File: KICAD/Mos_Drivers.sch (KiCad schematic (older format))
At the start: 15 parts, among them U12 UCC27284-Q1

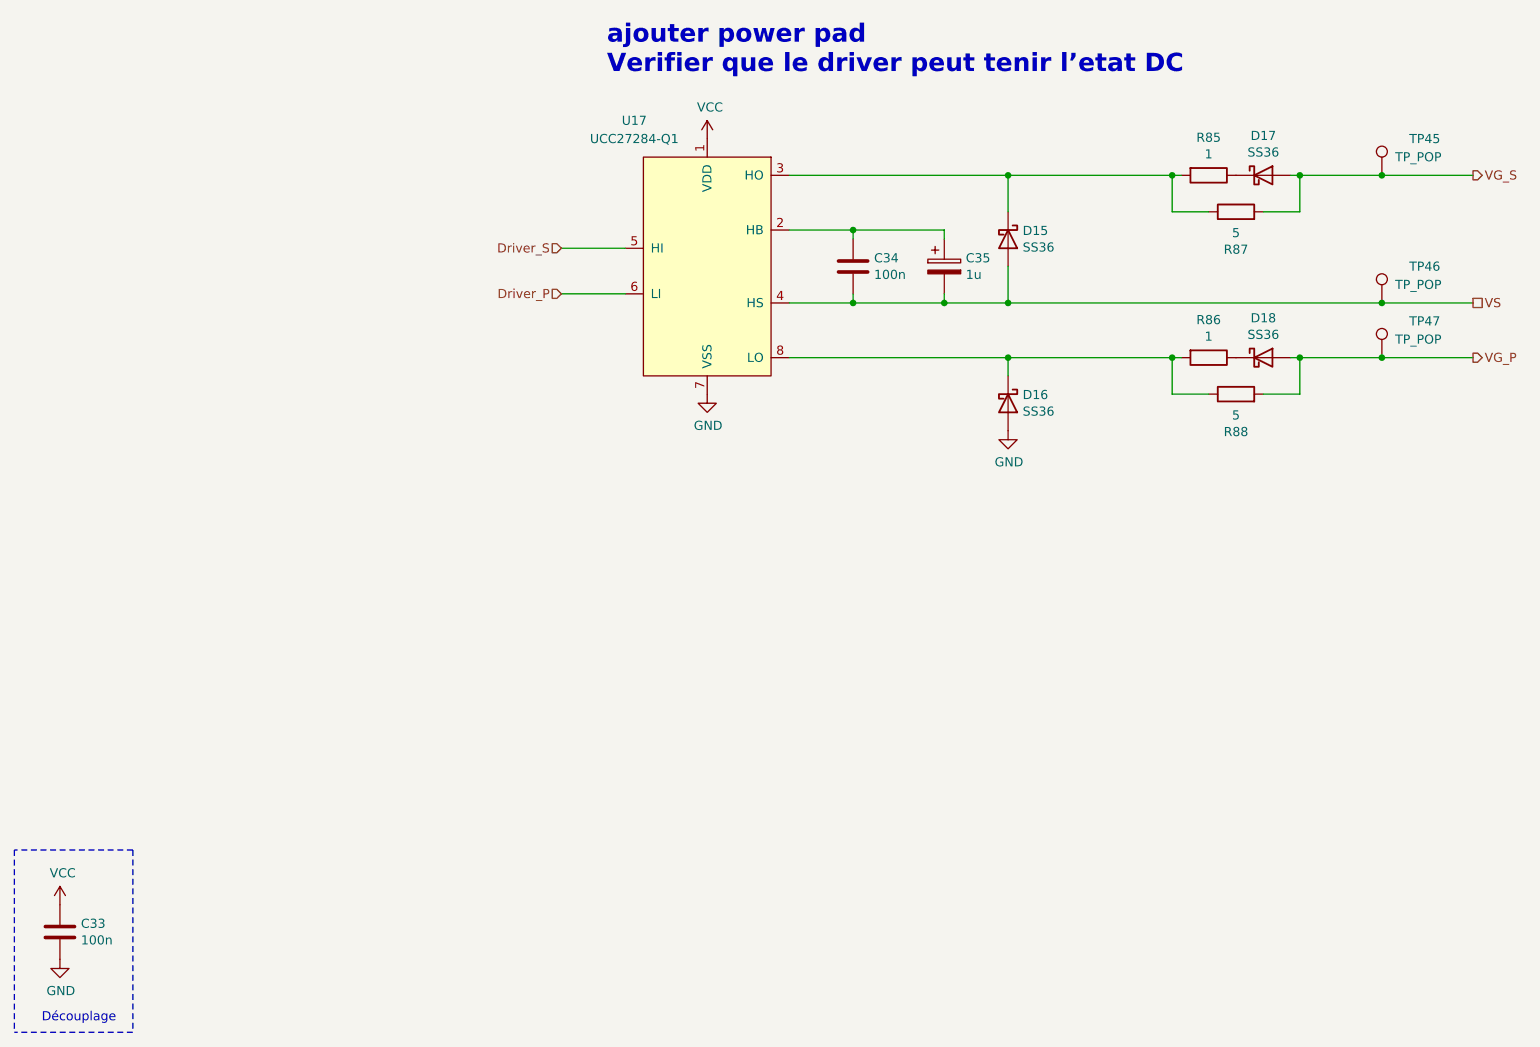
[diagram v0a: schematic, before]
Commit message: route + work on djd
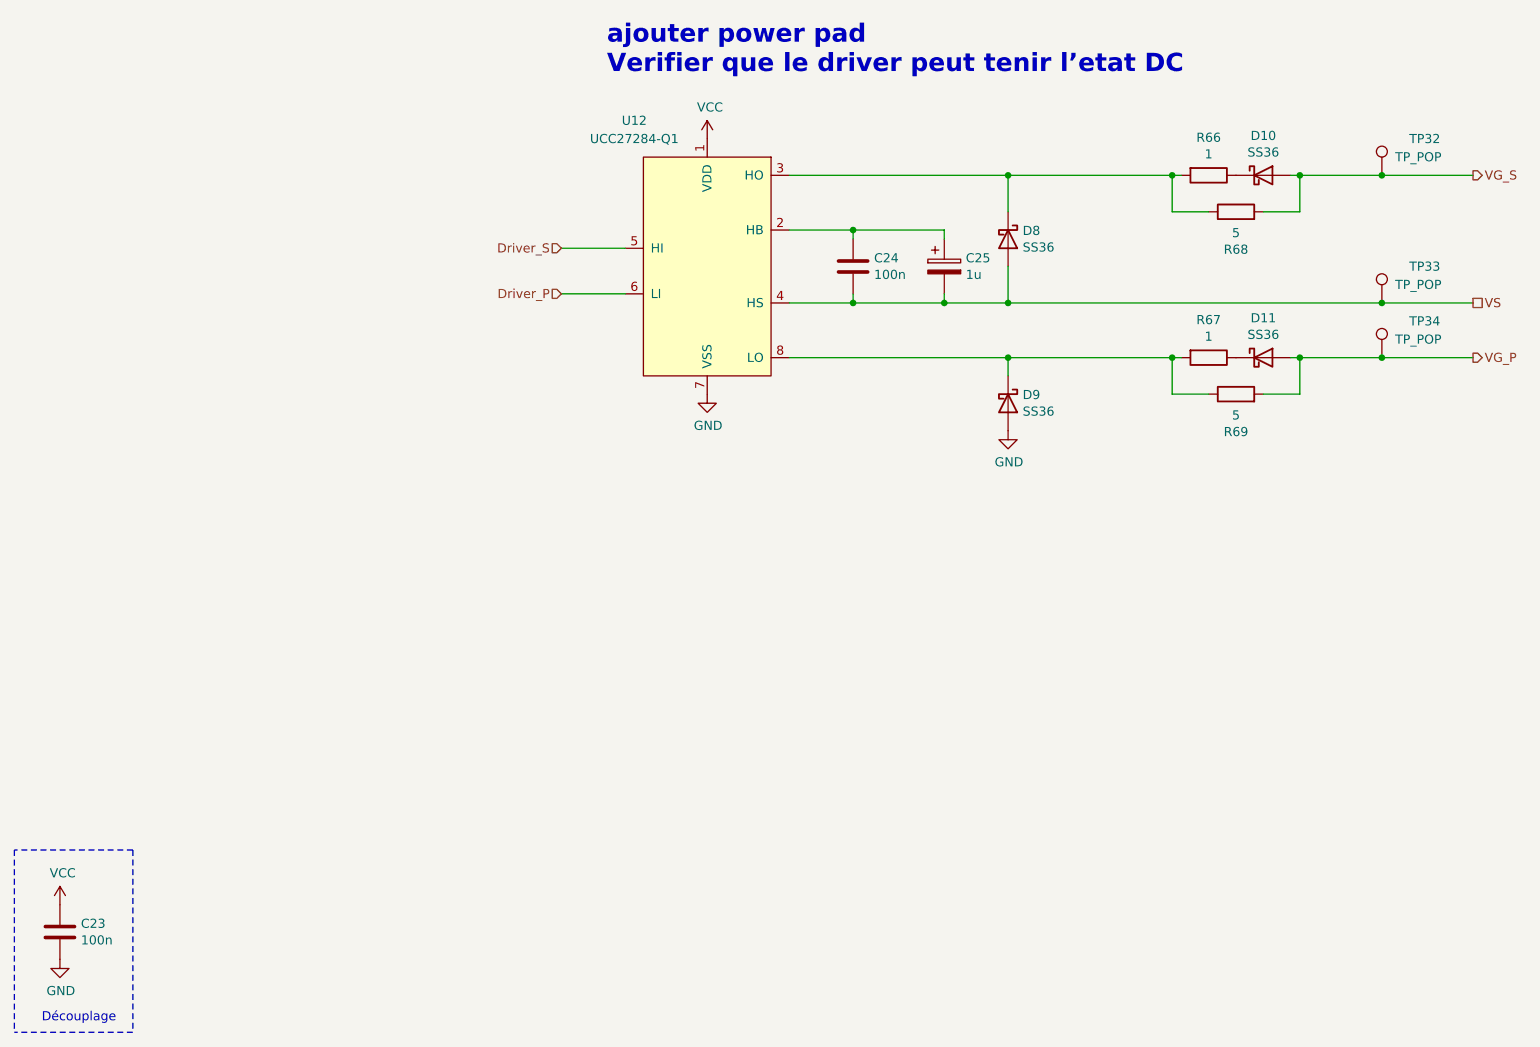
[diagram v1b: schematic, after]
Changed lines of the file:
@@
 $Descr A4 11693 8268
 encoding utf-8
-Sheet 16 17
+Sheet 12 17
 Title "SESAME"
 Date ""
@@
 AR Path="/61996C9F/612BC387" Ref="C?"  Part="1"
 AR Path="/619A00BB/612BC387" Ref="C33"  Part="1"
-F 0 "C33" H 965 7146 50  0000 L CNN
+F 0 "C23" H 965 7146 50  0000 L CNN
 F 1 "100n" H 965 7055 50  0000 L CNN
 F 2 "Capacitor_SMD:C_0805_2012Metric_Pad1.15x1.40mm_HandSolder" H 888 6950 50  0001 C CNN
@@
 AR Path="/61996C9F/612C31FB" Ref="D?"  Part="1"
 AR Path="/619A00BB/612C31FB" Ref="D15"  Part="1"
-F 0 "D15" V 6004 3380 50  0000 L CNN
+F 0 "D8" V 6004 3380 50  0000 L CNN
 F 1 "SS36" V 6095 3380 50  0000 L CNN
 F 2 "Diode_SMD:D_SMA_Handsoldering" H 6050 3300 50  0001 C CNN
@@
 AR Path="/61996C9F/6154F3B3" Ref="TP?"  Part="1"
 AR Path="/619A00BB/6154F3B3" Ref="TP46"  Part="1"
-F 0 "TP46" H 8250 3850 50  0000 L CNN
+F 0 "TP33" H 8250 3850 50  0000 L CNN
 F 1 "TP_POP" H 8300 3750 50  0000 C CNN
 F 2 "TestPoint:TestPoint_Loop_D1.80mm_Drill1.0mm_Beaded" H 8300 3650 50  0001 C CNN
@@
 AR Path="/61996C9F/61556ADA" Ref="TP?"  Part="1"
 AR Path="/619A00BB/61556ADA" Ref="TP47"  Part="1"
-F 0 "TP47" H 8250 4150 50  0000 L CNN
+F 0 "TP34" H 8250 4150 50  0000 L CNN
 F 1 "TP_POP" H 8300 4050 50  0000 C CNN
 F 2 "TestPoint:TestPoint_Loop_D1.80mm_Drill1.0mm_Beaded" H 8300 3950 50  0001 C CNN
@@
 AR Path="/61996C9F/61556D55" Ref="TP?"  Part="1"
 AR Path="/619A00BB/61556D55" Ref="TP45"  Part="1"
-F 0 "TP45" H 8250 3150 50  0000 L CNN
+F 0 "TP32" H 8250 3150 50  0000 L CNN
 F 1 "TP_POP" H 8300 3050 50  0000 C CNN
 F 2 "TestPoint:TestPoint_Loop_D1.80mm_Drill1.0mm_Beaded" H 8300 2950 50  0001 C CNN
@@
 AR Path="/61996C9F/615F8500" Ref="U?"  Part="1"
 AR Path="/619A00BB/615F8500" Ref="U17"  Part="1"
-F 0 "U17" H 4000 4250 50  0000 C CNN
+F 0 "U12" H 4000 4250 50  0000 C CNN
 F 1 "UCC27284-Q1" H 4000 4150 50  0000 C CNN
 F 2 "Package_SO:SOIC-8_3.9x4.9mm_P1.27mm" H 4400 3450 50  0001 C CNN
@@
 AR Path="/61996C9F/617A570A" Ref="D?"  Part="1"
 AR Path="/619A00BB/617A570A" Ref="D16"  Part="1"
-F 0 "D16" V 6004 4280 50  0000 L CNN
+F 0 "D9" V 6004 4280 50  0000 L CNN
 F 1 "SS36" V 6095 4280 50  0000 L CNN
 F 2 "Diode_SMD:D_SMA_Handsoldering" H 6050 4200 50  0001 C CNN
@@
 AR Path="/61996C9F/617B4129" Ref="D?"  Part="1"
 AR Path="/619A00BB/617B4129" Ref="D17"  Part="1"
-F 0 "D17" H 7450 3167 50  0000 C CNN
+F 0 "D10" H 7450 3167 50  0000 C CNN
 F 1 "SS36" H 7450 3076 50  0000 C CNN
 F 2 "Diode_SMD:D_SMA_Handsoldering" H 7450 2950 50  0001 C CNN
@@
 AR Path="/61996C9F/617C4D4F" Ref="R?"  Part="1"
 AR Path="/619A00BB/617C4D4F" Ref="R85"  Part="1"
-F 0 "R85" V 6943 2950 50  0000 C CNN
+F 0 "R66" V 6943 2950 50  0000 C CNN
 F 1 "1" V 7034 2950 50  0000 C CNN
 F 2 "Resistor_SMD:R_0805_2012Metric_Pad1.15x1.40mm_HandSolder" V 7080 2950 50  0001 C CNN
@@
 AR Path="/61996C9F/617CA6D6" Ref="R?"  Part="1"
 AR Path="/619A00BB/617CA6D6" Ref="R87"  Part="1"
-F 0 "R87" V 7093 3150 50  0000 C CNN
+F 0 "R68" V 7093 3150 50  0000 C CNN
 F 1 "5" V 7184 3150 50  0000 C CNN
 F 2 "Resistor_SMD:R_0805_2012Metric_Pad1.15x1.40mm_HandSolder" V 7230 3150 50  0001 C CNN
@@
 AR Path="/60F19D6C/619F44C6" Ref="C25"  Part="1"
 AR Path="/619A00BB/619F44C6" Ref="C35"  Part="1"
-F 0 "C35" H 5818 3496 50  0000 L CNN
+F 0 "C25" H 5818 3496 50  0000 L CNN
 F 1 "1u" H 5818 3405 50  0000 L CNN
 F 2 "Capacitor_SMD:C_0805_2012Metric_Pad1.15x1.40mm_HandSolder" H 5738 3300 50  0001 C CNN
@@
 AR Path="/61996C9F/61A058A4" Ref="D?"  Part="1"
 AR Path="/619A00BB/61A058A4" Ref="D18"  Part="1"
-F 0 "D18" H 7450 4167 50  0000 C CNN
+F 0 "D11" H 7450 4167 50  0000 C CNN
 F 1 "SS36" H 7450 4076 50  0000 C CNN
 F 2 "Diode_SMD:D_SMA_Handsoldering" H 7450 3950 50  0001 C CNN
@@
 AR Path="/61996C9F/61A058AA" Ref="R?"  Part="1"
 AR Path="/619A00BB/61A058AA" Ref="R86"  Part="1"
-F 0 "R86" V 6943 3950 50  0000 C CNN
+F 0 "R67" V 6943 3950 50  0000 C CNN
 F 1 "1" V 7034 3950 50  0000 C CNN
 F 2 "Resistor_SMD:R_0805_2012Metric_Pad1.15x1.40mm_HandSolder" V 7080 3950 50  0001 C CNN
@@
 AR Path="/61996C9F/61A058B0" Ref="R?"  Part="1"
 AR Path="/619A00BB/61A058B0" Ref="R88"  Part="1"
-F 0 "R88" V 7093 4150 50  0000 C CNN
+F 0 "R69" V 7093 4150 50  0000 C CNN
 F 1 "5" V 7184 4150 50  0000 C CNN
 F 2 "Resistor_SMD:R_0805_2012Metric_Pad1.15x1.40mm_HandSolder" V 7230 4150 50  0001 C CNN
@@
 AR Path="/61996C9F/61A06D05" Ref="C?"  Part="1"
 AR Path="/619A00BB/61A06D05" Ref="C34"  Part="1"
-F 0 "C34" H 5315 3496 50  0000 L CNN
+F 0 "C24" H 5315 3496 50  0000 L CNN
 F 1 "100n" H 5315 3405 50  0000 L CNN
 F 2 "Capacitor_SMD:C_0805_2012Metric_Pad1.15x1.40mm_HandSolder" H 5238 3300 50  0001 C CNN
